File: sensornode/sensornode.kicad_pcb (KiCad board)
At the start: 2 copper layers, 57.6 x 43.9 mm, 24 parts, among them J1 Conn_01x02, J2 Conn_01x06_Male, J3 Conn_01x04_Male, J4 USB_B_Micro, Q1 MMBT3904, U1 ESP-12F, U2 MQ-135, U3 LTC4055, U4 MIC5504-3.3YM5

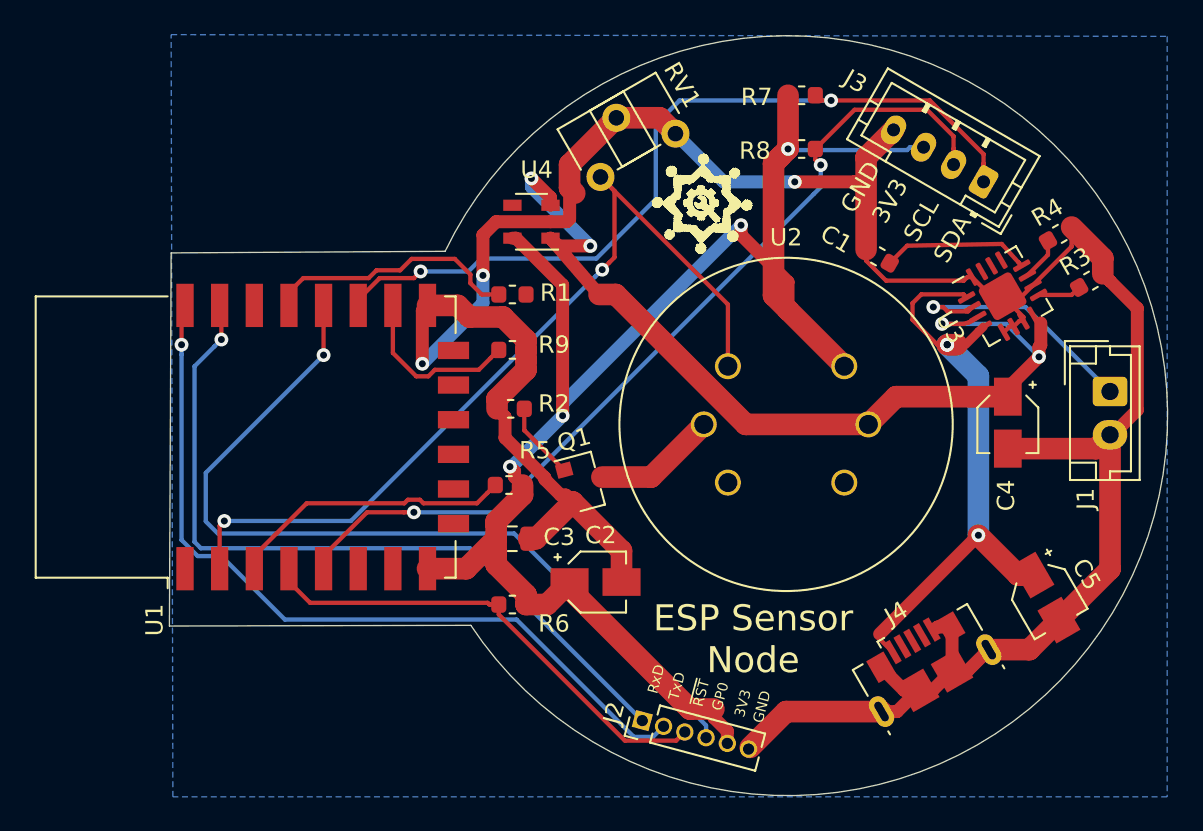
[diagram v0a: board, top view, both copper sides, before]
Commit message: update to latest
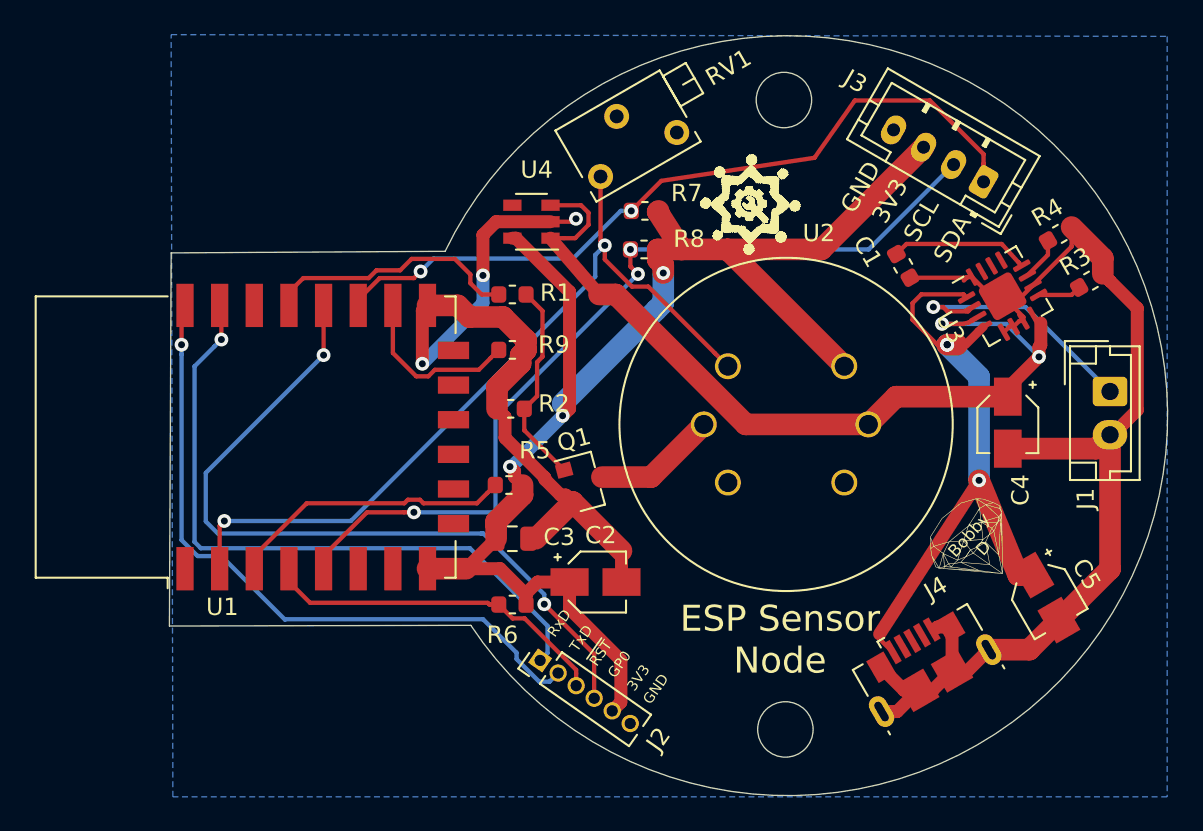
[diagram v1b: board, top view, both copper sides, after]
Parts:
- added G***: LOGO, logo:diamond, F.Cu at (201.8, 88.2)
- added REF**: MountingHole_3.2mm_M3, MountingHole:MountingHole_3.2mm_M3, F.Cu at (190.8, 62.7)
- added REF**: MountingHole_3.2mm_M3, MountingHole:MountingHole_3.2mm_M3, F.Cu at (190.9, 99.0)
- RV1: footprint Potentiometer_THT:Potentiometer_ACP_CA6-H2,5_Horizontal -> Potentiometer_THT:Potentiometer_Bourns_3266X_Horizontal
- moved R7 11.2 mm to (182.8, 69.1), turned to 180 degrees
- moved R8 10.8 mm to (182.7, 71.3), turned to 180 degrees
- moved J2 6.85 mm to (176.7, 95.0), turned to 55 degrees
- moved C1 1.56 mm to (197.7, 72.2), turned to 300 degrees
- turned RV1 to 210 degrees
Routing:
- net GND: track 157.3 -> 112.1 mm
- net +3V3: track 93.9 -> 84.4 mm, vias 4 -> 3
- net /~RST: track 27.9 -> 20.3 mm
- net Net-(Q1-Pad1): track 4.49 -> 11.9 mm
- net /TX: track 46.4 -> 39.2 mm
- net /GP0: track 49.8 -> 43.8 mm, vias 1 -> 2
- net /RX: track 44.5 -> 38.9 mm
- net +5V: track 55.7 -> 51.5 mm, vias 4 -> 2
- net /mq135_adc: track 50.6 -> 46.7 mm
- net /SDA: track 48.7 -> 45.0 mm
- net VBUS: track 35.3 -> 37.3 mm
- net /SCL: track 51.8 -> 51.2 mm, vias 2 -> 3
- net Net-(C1-Pad1): track 8.59 -> 8.03 mm
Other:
- board text added: "Bobby D"

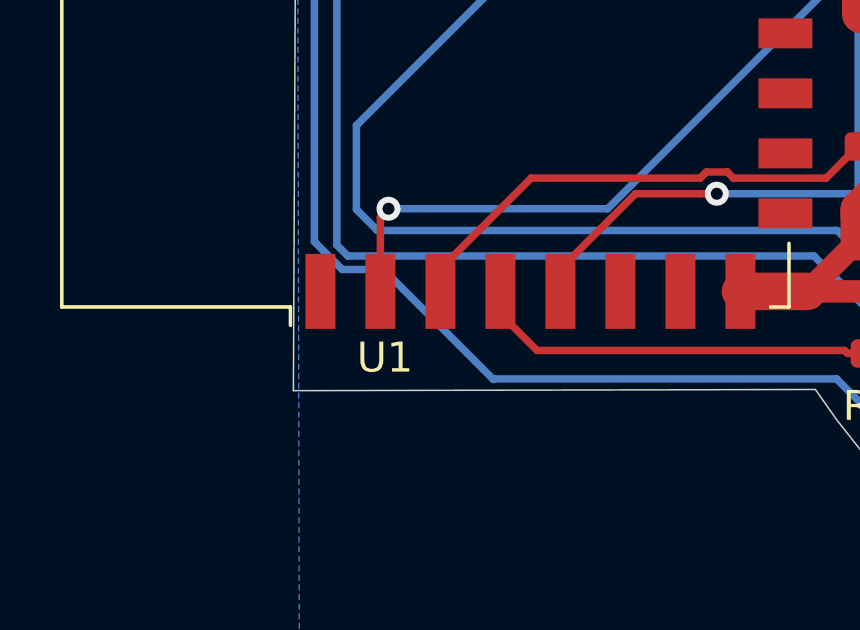
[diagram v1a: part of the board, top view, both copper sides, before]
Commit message: update board
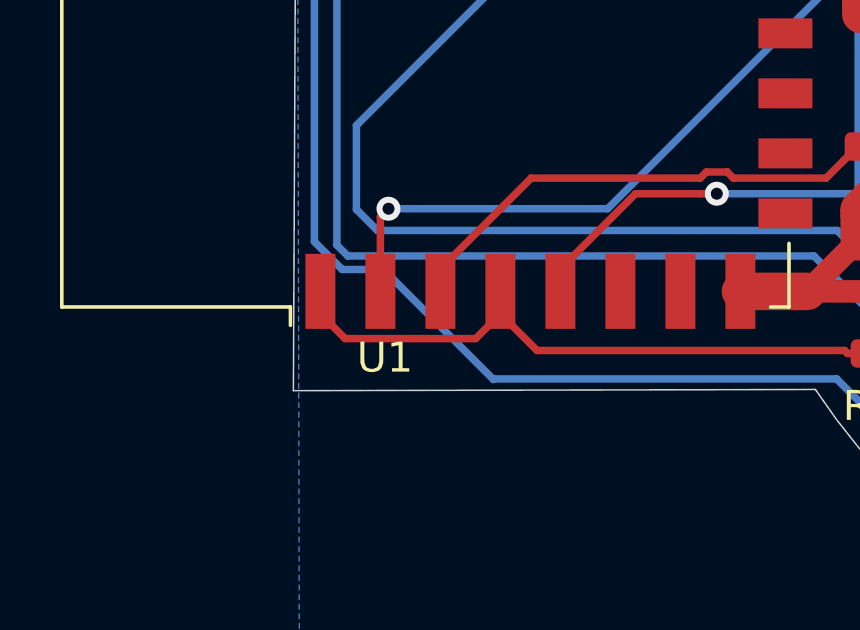
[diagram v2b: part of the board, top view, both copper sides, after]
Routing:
- net /~RST: track 20.3 -> 27.8 mm
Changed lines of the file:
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@@
     (thickness 1.6)
     (drawings 7964)
-    (tracks 305)
+    (tracks 309)
     (zones 0)
     (modules 27)
@@
   (page A4)
   (layers
-    (0 F.Cu signal hide)
-    (31 B.Cu signal hide)
+    (0 F.Cu signal)
+    (31 B.Cu signal)
     (32 B.Adhes user)
     (33 F.Adhes user)
@@
       (outputformat 1)
       (mirror false)
-      (drillshape 1)
+      (drillshape 0)
       (scaleselection 1)
       (outputdirectory ""))
@@
   (segment (start 173.408361 92.648362) (end 161.98686 92.648362) (width 0.25) (layer B.Cu) (net 12))
   (segment (start 175.34205 94.58205) (end 173.408361 92.648362) (width 0.25) (layer B.Cu) (net 12))
-  (segment (start 162.2 90.48) (end 162.2 89.73) (width 0.25) (layer F.Cu) (net 13))
   (segment (start 163.42 91.7) (end 162.2 90.48) (width 0.25) (layer F.Cu) (net 13))
   (segment (start 173.675 91.7) (end 163.42 91.7) (width 0.25) (layer F.Cu) (net 13))
@@
   (segment (start 175.11251 92.60001) (end 175.807893 92.60001) (width 0.25) (layer F.Cu) (net 13))
   (segment (start 174.3125 91.8) (end 175.11251 92.60001) (width 0.25) (layer F.Cu) (net 13))
+  (segment (start 162.2 90.48) (end 162.2 89.73) (width 0.25) (layer F.Cu) (net 13))
+  (segment (start 157.025001 91.305001) (end 161.374999 91.305001) (width 0.25) (layer F.Cu) (net 13))
+  (segment (start 156.2 90.48) (end 157.025001 91.305001) (width 0.25) (layer F.Cu) (net 13))
+  (segment (start 161.374999 91.305001) (end 162.2 90.48) (width 0.25) (layer F.Cu) (net 13))
+  (segment (start 156.2 89.73) (end 156.2 90.48) (width 0.25) (layer F.Cu) (net 13))
   (segment (start 158.1 87.7) (end 157.4 87) (width 0.25) (layer B.Cu) (net 14))
   (via (at 164.2 77.4) (size 0.8) (drill 0.4) (layers F.Cu B.Cu) (net 14))
